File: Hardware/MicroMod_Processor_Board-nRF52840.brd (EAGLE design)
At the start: 22 x 22 mm, 30 parts, among them J2 MICROMOD-2222, U1 W25QXX128MBIT-6X5, U2 MDBT50Q, Y1 32.768kHz

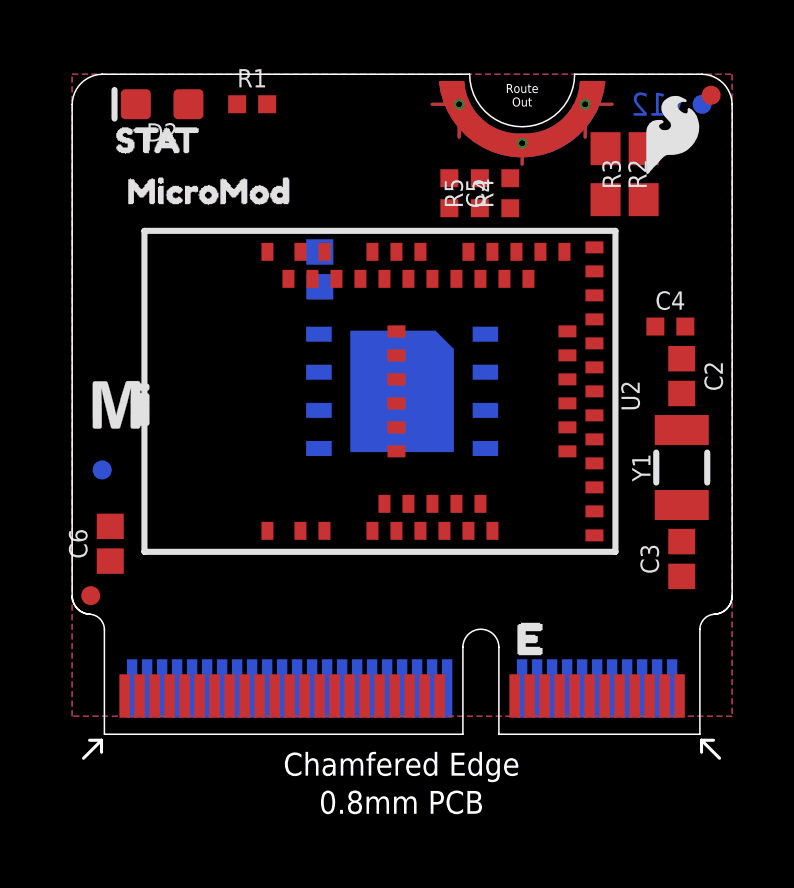
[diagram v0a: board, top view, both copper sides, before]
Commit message: Started routing
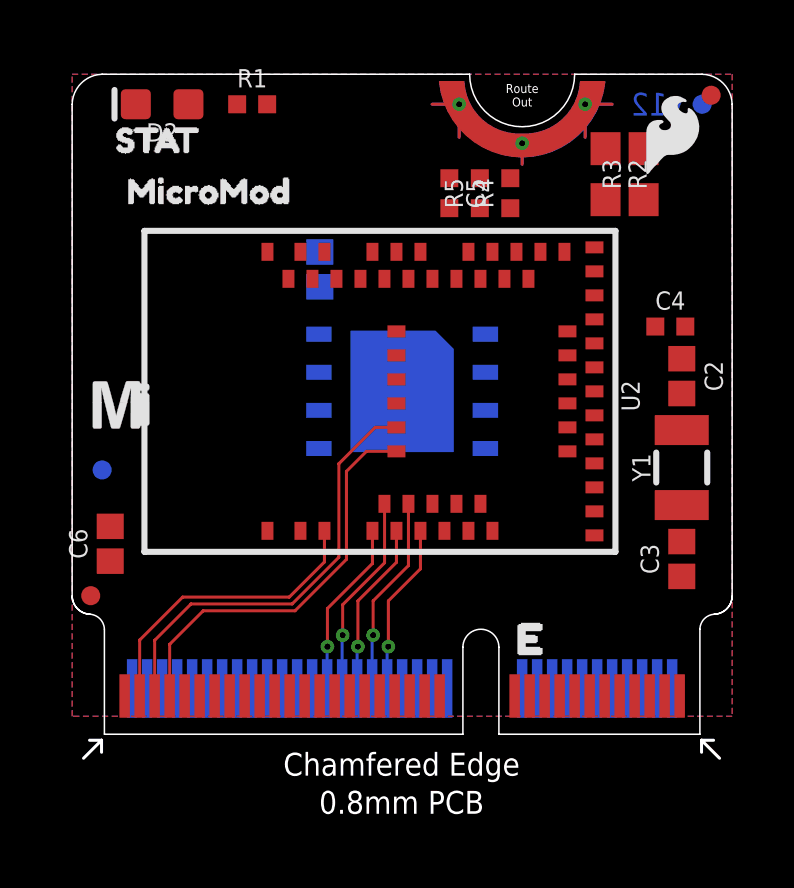
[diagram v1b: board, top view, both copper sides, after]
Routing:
- net GPIO6: track 0.00 -> 14.7 mm
- net GPIO7: track 0.00 -> 13.7 mm
- net GPIO5: track 0.00 -> 10.1 mm
- net GPIO3: track 0.00 -> 6.74 mm, vias 0 -> 1
- net GPIO1: track 0.00 -> 6.66 mm, vias 0 -> 1
- net GPIO4: track 0.00 -> 5.88 mm, vias 0 -> 1
- net GPIO2: track 0.00 -> 5.80 mm, vias 0 -> 1
- net GPIO0: track 0.00 -> 5.71 mm, vias 0 -> 1
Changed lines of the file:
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@@
 </class>
 </classes>
-<designrules name="SparkFun-4-layer-MicroMod">
-<description language="en">&lt;b&gt;SparkFun 2 Layer Design Rule Checks - Limits for PCBWay&lt;/b&gt;
+<designrules name="SparkFun-4-layer-FAB-LIMIT">
+<description language="en">&lt;b&gt;EAGLE Design Rules&lt;/b&gt;
 &lt;p&gt;
- If you're ordering from PCBWay, these are the 'free' minimums.</description>
-<param name="layerSetup" value="(1+2*15+16)"/>
-<param name="mtCopper" value="0.035mm 0.035mm 0.035mm 0.035mm 0.035mm 0.035mm 0.035mm 0.035mm 0.035mm 0.035mm 0.035mm 0.035mm 0.035mm 0.035mm 0.035mm 0.035mm"/>
-<param name="mtIsolate" value="1.5mm 0.15mm 0.2mm 0.15mm 0.2mm 0.15mm 0.2mm 0.15mm 0.2mm 0.15mm 0.2mm 0.15mm 0.2mm 0.15mm 0.2mm"/>
-<param name="mdWireWire" value="4mil"/>
-<param name="mdWirePad" value="4mil"/>
-<param name="mdWireVia" value="4mil"/>
-<param name="mdPadPad" value="4mil"/>
-<param name="mdPadVia" value="4mil"/>
-<param name="mdViaVia" value="4mil"/>
-<param name="mdSmdPad" value="4mil"/>
-<param name="mdSmdVia" value="4mil"/>
-<param name="mdSmdSmd" value="4mil"/>
+The default Design Rules have been set to cover
+a wide range of applications. Your particular design
+may have different requirements, so please make the
+necessary adjustments and save your customized
+design rules under a new name.</description>
+<param name="layerSetup" value="(1*2*15*16)"/>
+<param name="mtCopper" value="0.035559375mm 0.035559375mm 0.035mm 0.035mm 0.035mm 0.035mm 0.035mm 0.035mm 0.035mm 0.035mm 0.035mm 0.035mm 0.035mm 0.035mm 0.035559375mm 0.035559375mm"/>
+<param name="mtIsolate" value="0.47751875mm 0.47751875mm 0.2mm 0.15mm 0.2mm 0.15mm 0.2mm 0.15mm 0.2mm 0.15mm 0.2mm 0.15mm 0.2mm 0.15mm 0.47751875mm"/>
+<param name="mdWireWire" value="5mil"/>
+<param name="mdWirePad" value="5mil"/>
+<param name="mdWireVia" value="5mil"/>
+<param name="mdPadPad" value="5mil"/>
+<param name="mdPadVia" value="5mil"/>
+<param name="mdViaVia" value="5mil"/>
+<param name="mdSmdPad" value="5mil"/>
+<param name="mdSmdVia" value="5mil"/>
+<param name="mdSmdSmd" value="5mil"/>
 <param name="mdViaViaSameLayer" value="8mil"/>
 <param name="mnLayersViaInSmd" value="2"/>
-<param name="mdCopperDimension" value="6mil"/>
-<param name="mdDrill" value="6mil"/>
+<param name="mdCopperDimension" value="4mil"/>
+<param name="mdDrill" value="4mil"/>
 <param name="mdSmdStop" value="0mil"/>
 <param name="msWidth" value="4mil"/>
-<param name="msDrill" value="0.2mm"/>
+<param name="msDrill" value="6mil"/>
 <param name="msMicroVia" value="9.99mm"/>
 <param name="msBlindViaRatio" value="0.5"/>
@@
 <param name="rvMicroViaOuter" value="0.25"/>
 <param name="rvMicroViaInner" value="0.25"/>
-<param name="rlMinPadTop" value="3mil"/>
+<param name="rlMinPadTop" value="5mil"/>
 <param name="rlMaxPadTop" value="20mil"/>
-<param name="rlMinPadInner" value="3mil"/>
+<param name="rlMinPadInner" value="6mil"/>
 <param name="rlMaxPadInner" value="20mil"/>
-<param name="rlMinPadBottom" value="3mil"/>
+<param name="rlMinPadBottom" value="5mil"/>
 <param name="rlMaxPadBottom" value="20mil"/>
-<param name="rlMinViaOuter" value="3mil"/>
+<param name="rlMinViaOuter" value="5mil"/>
 <param name="rlMaxViaOuter" value="20mil"/>
-<param name="rlMinViaInner" value="3mil"/>
+<param name="rlMinViaInner" value="6mil"/>
 <param name="rlMaxViaInner" value="20mil"/>
-<param name="rlMinMicroViaOuter" value="3mil"/>
+<param name="rlMinMicroViaOuter" value="4mil"/>
 <param name="rlMaxMicroViaOuter" value="20mil"/>
-<param name="rlMinMicroViaInner" value="3mil"/>
+<param name="rlMinMicroViaInner" value="4mil"/>
 <param name="rlMaxMicroViaInner" value="20mil"/>
 <param name="psTop" value="-1"/>
@@
 <contactref element="J2" pad="73"/>
 <contactref element="U2" pad="3"/>
-<wire x1="2.25" y1="1.275" x2="8.41" y2="6.78" width="0" layer="19" extent="1-1"/>
+<wire x1="2.25" y1="1.275" x2="2.25" y2="3.139" width="0.1016" layer="1"/>
+<wire x1="8.41" y1="5.743" x2="8.41" y2="6.78" width="0.1016" layer="1"/>
+<wire x1="2.25" y1="3.139" x2="3.683" y2="4.572" width="0.1016" layer="1"/>
+<wire x1="3.683" y1="4.572" x2="7.239" y2="4.572" width="0.1016" layer="1"/>
+<wire x1="7.239" y1="4.572" x2="8.41" y2="5.743" width="0.1016" layer="1"/>
 </signal>
 <signal name="GPIO7">
 <contactref element="J2" pad="69"/>
 <contactref element="U2" pad="56"/>
-<wire x1="3.25" y1="1.275" x2="10.81" y2="9.43" width="0" layer="19" extent="1-1"/>
+<wire x1="3.25" y1="1.275" x2="3.25" y2="2.996" width="0.1016" layer="1"/>
+<wire x1="7.4283875" y1="4.1148" x2="9.144" y2="5.8304125" width="0.1016" layer="1"/>
+<wire x1="9.811" y1="9.43" x2="10.81" y2="9.43" width="0.1016" layer="1"/>
+<wire x1="3.25" y1="2.996" x2="4.3688" y2="4.1148" width="0.1016" layer="1"/>
+<wire x1="4.3688" y1="4.1148" x2="7.4283875" y2="4.1148" width="0.1016" layer="1"/>
+<wire x1="9.144" y1="5.8304125" x2="9.144" y2="8.763" width="0.1016" layer="1"/>
+<wire x1="9.144" y1="8.763" x2="9.811" y2="9.43" width="0.1016" layer="1"/>
 </signal>
 <signal name="GPIO6">
 <contactref element="J2" pad="71"/>
 <contactref element="U2" pad="57"/>
-<wire x1="2.75" y1="1.275" x2="10.81" y2="10.23" width="0" layer="19" extent="1-1"/>
+<wire x1="2.75" y1="1.275" x2="2.75" y2="3.131" width="0.1016" layer="1"/>
+<wire x1="3.9624" y1="4.3434" x2="7.33369375" y2="4.3434" width="0.1016" layer="1"/>
+<wire x1="7.33369375" y1="4.3434" x2="8.89" y2="5.89970625" width="0.1016" layer="1"/>
+<wire x1="8.89" y1="5.89970625" x2="8.89" y2="9.017" width="0.1016" layer="1"/>
+<wire x1="8.89" y1="9.017" x2="10.103" y2="10.23" width="0.1016" layer="1"/>
+<wire x1="10.103" y1="10.23" x2="10.81" y2="10.23" width="0.1016" layer="1"/>
+<wire x1="2.75" y1="3.131" x2="3.9624" y2="4.3434" width="0.1016" layer="1"/>
 </signal>
 <signal name="N$2">
@@
 <contactref element="J2" pad="42"/>
 <contactref element="U2" pad="7"/>
-<wire x1="10" y1="1.525" x2="11.21" y2="7.68" width="0" layer="19" extent="1-16"/>
+<wire x1="10" y1="1.525" x2="10" y2="3.269" width="0.1016" layer="16"/>
+<wire x1="10" y1="3.269" x2="10.033" y2="3.302" width="0.1016" layer="16"/>
+<via x="10.033" y="3.302" extent="1-16" drill="0.2032"/>
+<wire x1="10.033" y1="3.302" x2="10.033" y2="4.445" width="0.1016" layer="1"/>
+<wire x1="11.21" y1="5.622" x2="11.21" y2="7.68" width="0.1016" layer="1"/>
+<wire x1="10.033" y1="4.445" x2="11.21" y2="5.622" width="0.1016" layer="1"/>
 </signal>
 <signal name="GPIO3">
 <contactref element="J2" pad="46"/>
 <contactref element="U2" pad="5"/>
-<wire x1="9" y1="1.525" x2="10.41" y2="7.68" width="0" layer="19" extent="1-16"/>
+<wire x1="9" y1="1.525" x2="9" y2="3.285" width="0.1016" layer="16"/>
+<wire x1="9" y1="3.285" x2="9.017" y2="3.302" width="0.1016" layer="16"/>
+<via x="9.017" y="3.302" extent="1-16" drill="0.2032"/>
+<wire x1="9.017" y1="3.302" x2="9.017" y2="4.318" width="0.1016" layer="1"/>
+<wire x1="9.017" y1="4.318" x2="10.414" y2="5.715" width="0.1016" layer="1"/>
+<wire x1="10.414" y1="5.715" x2="10.414" y2="7.676" width="0.1016" layer="1"/>
+<wire x1="10.414" y1="7.676" x2="10.41" y2="7.68" width="0.1016" layer="1"/>
 </signal>
 <signal name="GPIO2">
 <contactref element="J2" pad="44"/>
 <contactref element="U2" pad="6"/>
-<wire x1="9.5" y1="1.525" x2="10.81" y2="6.78" width="0" layer="19" extent="1-16"/>
+<wire x1="9.5" y1="1.525" x2="9.5" y2="2.896" width="0.1016" layer="16"/>
+<wire x1="9.5" y1="2.896" x2="9.525" y2="2.921" width="0.1016" layer="16"/>
+<via x="9.525" y="2.921" extent="1-16" drill="0.2032"/>
+<wire x1="9.525" y1="2.921" x2="9.525" y2="4.445" width="0.1016" layer="1"/>
+<wire x1="10.81" y1="5.73" x2="10.81" y2="6.78" width="0.1016" layer="1"/>
+<wire x1="9.525" y1="4.445" x2="10.81" y2="5.73" width="0.1016" layer="1"/>
 </signal>
 <signal name="GPIO4">
 <contactref element="J2" pad="48"/>
 <contactref element="U2" pad="4"/>
-<wire x1="8.5" y1="1.525" x2="10.01" y2="6.78" width="0" layer="19" extent="1-16"/>
+<wire x1="8.5" y1="1.525" x2="8.5" y2="2.912" width="0.1016" layer="16"/>
+<wire x1="8.5" y1="2.912" x2="8.509" y2="2.921" width="0.1016" layer="16"/>
+<via x="8.509" y="2.921" extent="1-16" drill="0.2032"/>
+<wire x1="8.509" y1="2.921" x2="8.509" y2="4.191" width="0.1016" layer="1"/>
+<wire x1="10.01" y1="5.692" x2="10.01" y2="6.78" width="0.1016" layer="1"/>
+<wire x1="8.509" y1="4.191" x2="10.01" y2="5.692" width="0.1016" layer="1"/>
 </signal>
 <signal name="GPIO0">
 <contactref element="J2" pad="40"/>
 <contactref element="U2" pad="8"/>
-<wire x1="10.5" y1="1.525" x2="11.61" y2="6.78" width="0" layer="19" extent="1-16"/>
+<wire x1="10.5" y1="1.525" x2="10.5" y2="2.88" width="0.1016" layer="16"/>
+<wire x1="10.5" y1="2.88" x2="10.541" y2="2.921" width="0.1016" layer="16"/>
+<via x="10.541" y="2.921" extent="1-16" drill="0.2032"/>
+<wire x1="10.541" y1="2.921" x2="10.541" y2="4.445" width="0.1016" layer="1"/>
+<wire x1="11.61" y1="5.514" x2="11.61" y2="6.78" width="0.1016" layer="1"/>
+<wire x1="10.541" y1="4.445" x2="11.61" y2="5.514" width="0.1016" layer="1"/>
 </signal>
 <signal name="N$1">

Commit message: Routing
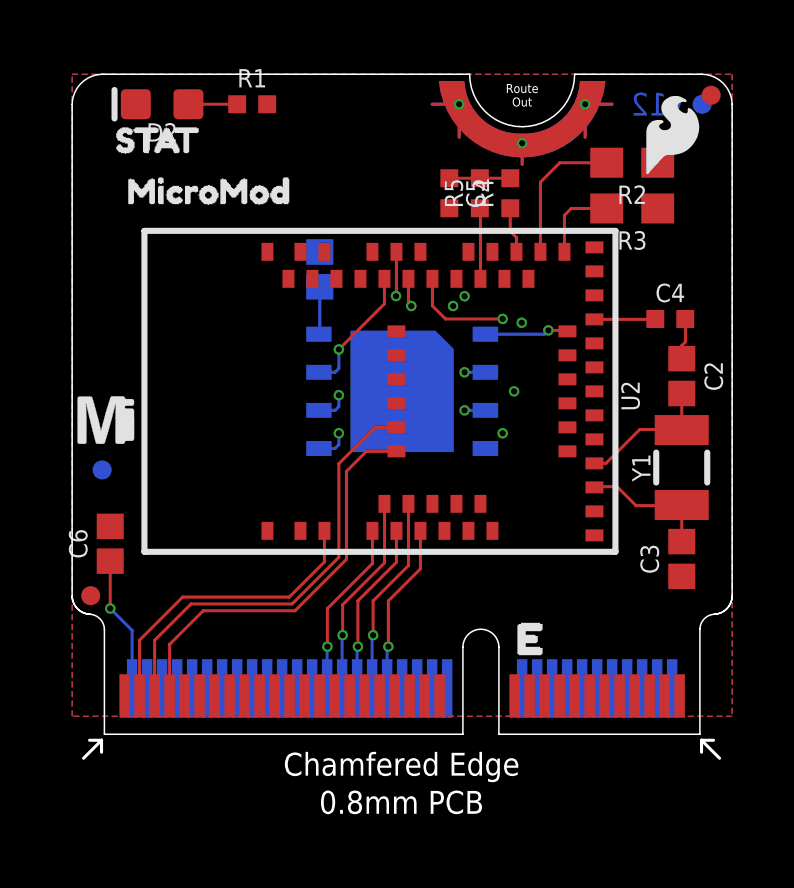
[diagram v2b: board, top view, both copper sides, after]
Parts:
- moved R3 1.20 mm to (18.7, 17.5), turned to 180 degrees
- moved R2 0.97 mm to (18.7, 19.1), turned to 180 degrees
- moved U$1 0.72 mm to (1.09, 10.5)
- moved C4 0.25 mm to (19.9, 13.8)
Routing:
- net SPI_MISO: track 0.00 -> 13.8 mm, vias 0 -> 3
- net 3.3V: track 0.00 -> 10.2 mm, vias 0 -> 1
- net SPI_SCK: track 0.00 -> 9.38 mm, vias 0 -> 3
- net SDIO_DATA1: track 0.00 -> 7.00 mm, vias 0 -> 3
- net SDIO_DATA2: track 0.00 -> 6.67 mm, vias 0 -> 3
- net N$1: track 0.00 -> 4.80 mm
- net N$5: track 0.00 -> 4.60 mm
- net N$4: track 0.00 -> 4.41 mm
- net SPI_!CS!: track 0.00 -> 4.34 mm, vias 0 -> 1
- net FLASH_!CS!: track 0.00 -> 2.80 mm, vias 0 -> 1
- net N$3: track 0.00 -> 2.72 mm
- net !RESET!: track 0.00 -> 2.36 mm
- net N$2: track 0.00 -> 1.62 mm
- net !BOOT!: track 0.00 -> 1.54 mm
- net GND: track 0.00 -> 1.38 mm
